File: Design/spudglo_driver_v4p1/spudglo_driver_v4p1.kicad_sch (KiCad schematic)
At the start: 20 parts, among them U10 receiver_433MHz, U11 receiver_433MHz, U5 receiver_433MHz, U7 PS2501-4, U8 TXS0104EDR, U9 receiver_433MHz

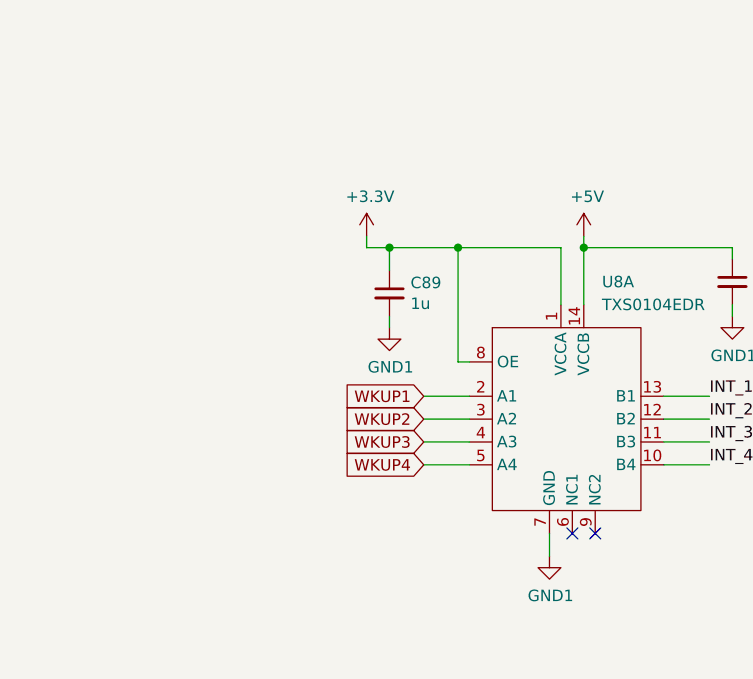
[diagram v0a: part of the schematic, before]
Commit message: spudglo v4p2!!!
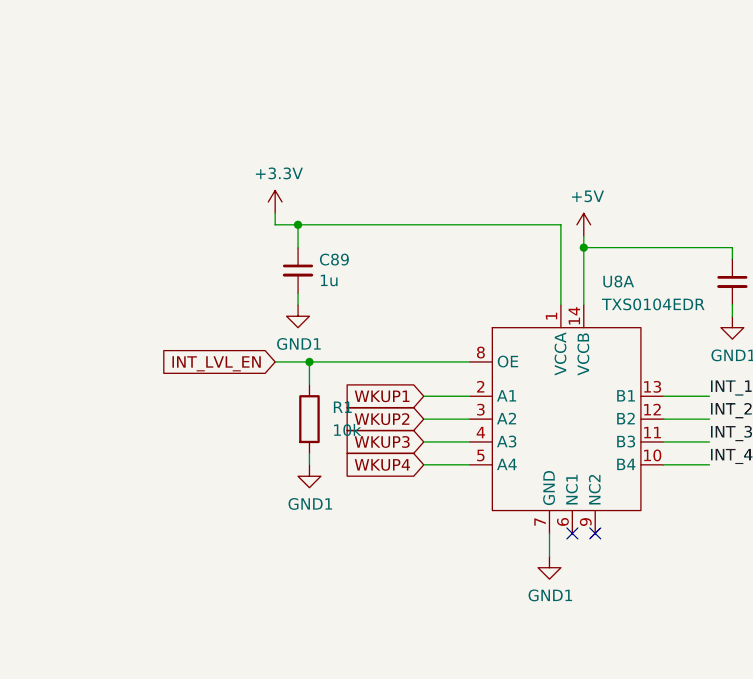
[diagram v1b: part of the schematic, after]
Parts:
- added R1: 10k, Resistor_SMD:R_0603_1608Metric_Pad0.98x0.95mm_HandSolder, symbol Device:R
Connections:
- net +3V3: no longer U8.8 (OE)
- net GND1: now also R1.2
- new net INT_LVL_EN: R1.1, U8.8 (OE)
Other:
- moved on the sheet: C89
